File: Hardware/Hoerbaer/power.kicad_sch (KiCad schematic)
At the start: 63 parts, among them J10 Battery 1S Li-Ion, J12 Battery 1S Li-Ion, Q1 DMG3415UQ-7, U12 MAX17048G, U13 TPS61288, U8 MCP73831T-2ACI/OT (4.2V), U9 TPS63001

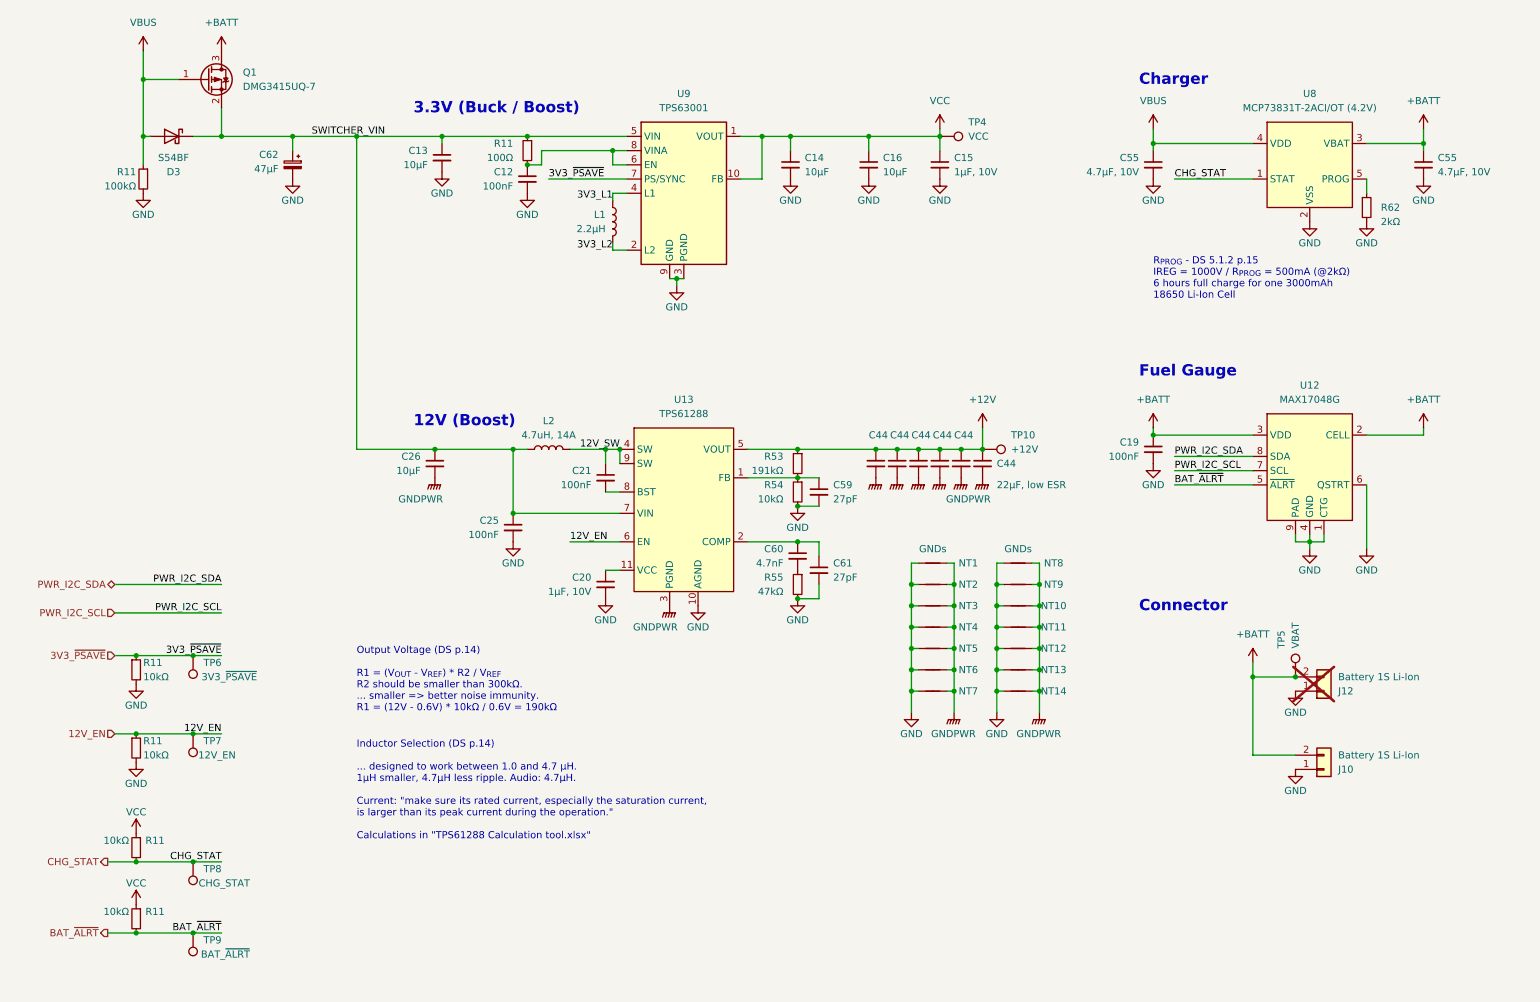
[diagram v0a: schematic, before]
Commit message: WIP new hw rev
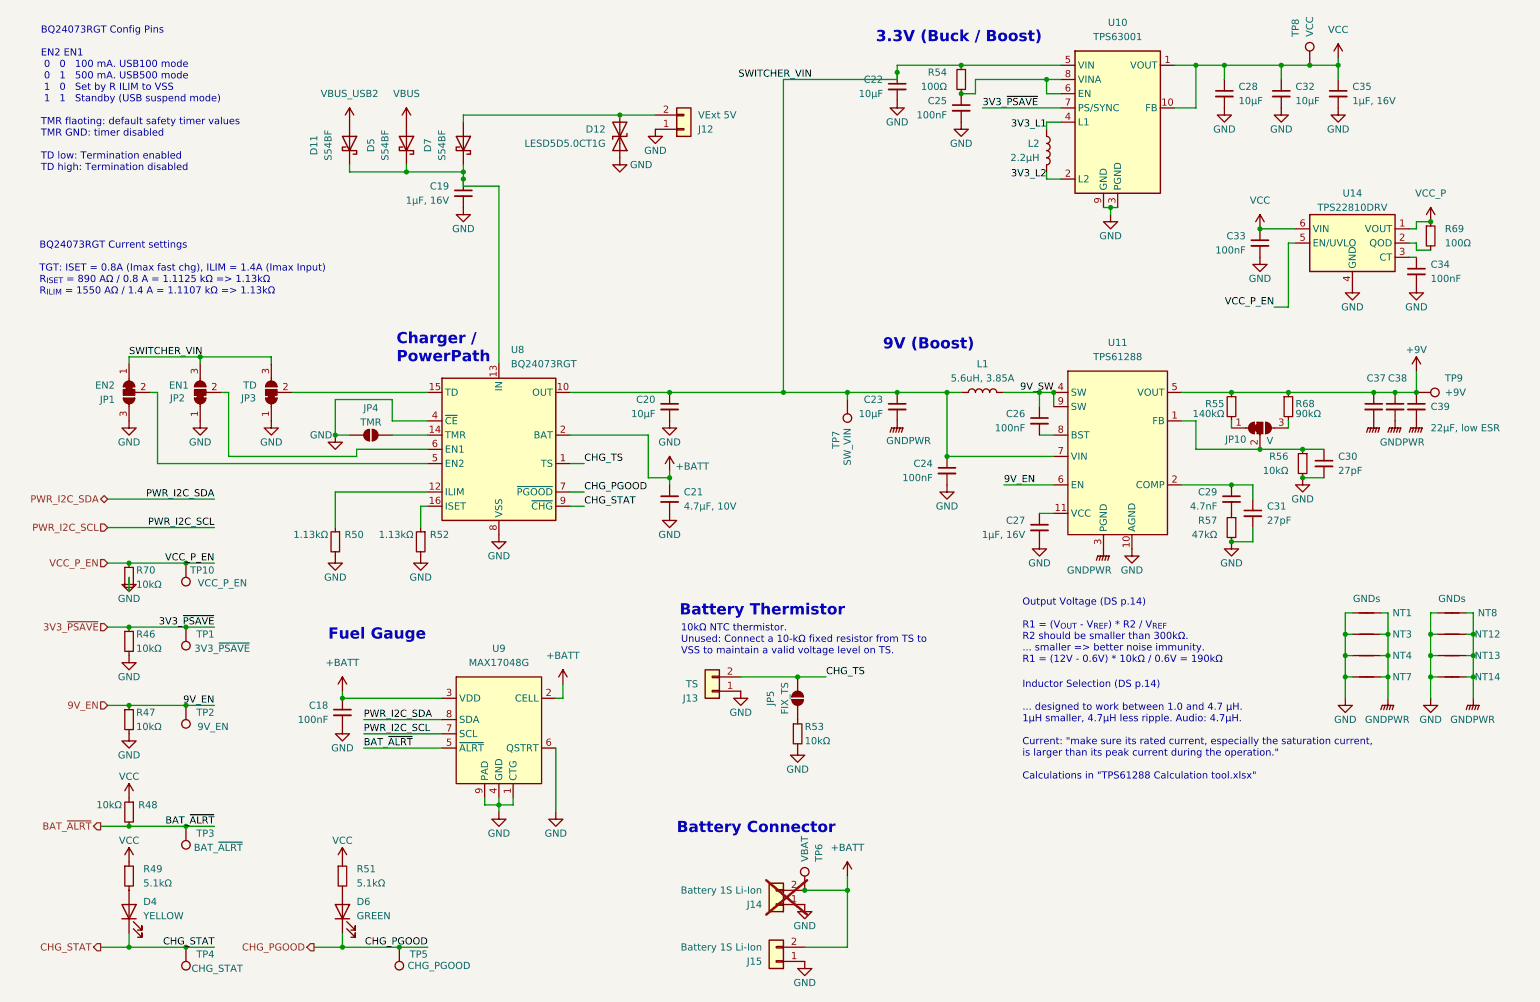
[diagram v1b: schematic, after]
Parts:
- removed C44 (x3): 22µF, low ESR, Capacitor_SMD:C_1210_3225Metric, symbol Device:C_Small
- removed C55: 4.7µF, 10V, Capacitor_SMD:C_0805_2012Metric, symbol Device:C_Small
- removed C62: 47µF, Capacitor_SMD:CP_Elec_6.3x5.9, symbol Device:C_Polarized_Small
- removed NT10, NT11, NT2, NT5, NT6, NT9: GNDs, Baer_Footprints:NetTie-2_Via, symbol Device:NetTie_2
- removed Q1: DMG3415UQ-7, Package_TO_SOT_SMD:SOT-23, symbol Device:Q_PMOS_GSD
- removed R11: 10kΩ, Resistor_SMD:R_0402_1005Metric, symbol Device:R_Small
- removed R11: 100kΩ, Resistor_SMD:R_0402_1005Metric, symbol Device:R_Small
- removed R62: 2kΩ, Resistor_SMD:R_0402_1005Metric, symbol Device:R_Small
- removed U8: MCP73831T-2ACI/OT (4.2V), Package_TO_SOT_SMD:SOT-23-5, symbol Baer_Symbols:MCP73831/2_SOT
- added C19: 1µF, 16V, Capacitor_SMD:C_0402_1005Metric, symbol Device:C_Small
- added C20: 10µF, Capacitor_SMD:C_0805_2012Metric, symbol Device:C_Small
- added C33, C34: 100nF, Capacitor_SMD:C_0402_1005Metric, symbol Device:C_Small
- added D11, D5: S54BF, Baer_Footprints:S54BF, symbol Device:D_Schottky
- added D12: LESD5D5.0CT1G, Diode_SMD:D_SOD-523, symbol Device:D_TVS
- added D4: YELLOW, LED_SMD:LED_0603_1608Metric, symbol Device:LED
- added D6: GREEN, LED_SMD:LED_0603_1608Metric, symbol Device:LED
- added J12: VExt 5V, Connector_Wire:SolderWire-0.5sqmm_1x02_P4.6mm_D0.9mm_OD2.1mm, symbol Connector_Generic:Conn_01x02
- added J13: TS, Connector_PinHeader_2.54mm:PinHeader_1x02_P2.54mm_Vertical, symbol Connector_Generic:Conn_01x02
- added JP1: EN2, Jumper:SolderJumper-3_P1.3mm_Bridged12_RoundedPad1.0x1.5mm, symbol Jumper:SolderJumper_3_Bridged12
- added JP10: V, Jumper:SolderJumper-3_P1.3mm_Bridged12_RoundedPad1.0x1.5mm, symbol Jumper:SolderJumper_3_Bridged12
- added JP2: EN1, Jumper:SolderJumper-3_P1.3mm_Bridged12_RoundedPad1.0x1.5mm, symbol Jumper:SolderJumper_3_Bridged12
- added JP3: TD, Jumper:SolderJumper-3_P1.3mm_Bridged12_RoundedPad1.0x1.5mm, symbol Jumper:SolderJumper_3_Bridged12
- added JP4: TMR, Jumper:SolderJumper-2_P1.3mm_Open_RoundedPad1.0x1.5mm, symbol Jumper:SolderJumper_2_Open
- added JP5: FIX_TS, Jumper:SolderJumper-2_P1.3mm_Open_RoundedPad1.0x1.5mm, symbol Jumper:SolderJumper_2_Open
- added R49, R51: 5.1kΩ, Resistor_SMD:R_0402_1005Metric, symbol Device:R_Small
- added R50, R52: 1.13kΩ, Resistor_SMD:R_0402_1005Metric, symbol Device:R_Small
- added R53, R70: 10kΩ, Resistor_SMD:R_0402_1005Metric, symbol Device:R_Small
- added R68: 90kΩ, Resistor_SMD:R_0402_1005Metric, symbol Device:R_Small
- added R69: 100Ω, Resistor_SMD:R_0402_1005Metric, symbol Device:R_Small
- added TP10: VCC_P_EN, TestPoint:TestPoint_Pad_D1.5mm, symbol Connector:TestPoint
- added TP5: CHG_PGOOD, TestPoint:TestPoint_Pad_D1.5mm, symbol Connector:TestPoint
- added TP7: SW_VIN, TestPoint:TestPoint_Pad_D1.5mm, symbol Connector:TestPoint
- added U14: TPS22810DRV, Package_SON:WSON-6-1EP_2x2mm_P0.65mm_EP1x1.6mm_ThermalVias, symbol Power_Management:TPS22810DRV
- added U8: BQ24073RGT, Package_DFN_QFN:VQFN-16-1EP_3x3mm_P0.5mm_EP1.6x1.6mm, symbol Battery_Management:BQ24073RGT
- C27: renamed from C20; value 1µF, 10V -> 1µF, 16V; LCSC C29266 -> C29266
- C35: renamed from C15; value 1µF, 10V -> 1µF, 16V; LCSC C29266 -> C29266
- L1: renamed from L2; value 4.7uH, 14A -> 5.6uH, 3.85A; footprint Baer_Footprints:L_TDK_SPM12565 -> Inductor_SMD:L_Sunlord_SWPA8040S; LCSC C2048059 -> C96972; MPN SPM12565VT-4R7M-D Copy -> SWPA8040S5R6NT
- R55: renamed from R53; value 191kΩ -> 140kΩ; LCSC C270632 -> C114151; MPN 0402WGF1913TCE -> RC0402FR-07140KL
- TP2: renamed from TP7; value 12V_EN -> 9V_EN
- TP9: renamed from TP10; value +12V -> +9V
- renumbered C19 to C18, C55 to C21, C13 to C22, C26 to C23, C25 to C24, C12 to C25, C21 to C26, C14 to C28, C60 to C29, C59 to C30, C61 to C31, C16 to C32, C44 to C37, C44 to C38, C44 to C39, D3 to D7, J12 to J14, J10 to J15, L1 to L2, R11 to R46, R11 to R47, R11 to R48, R11 to R54, R54 to R56, R55 to R57, TP6 to TP1, TP9 to TP3, TP8 to TP4, TP5 to TP6, TP4 to TP8, U9 to U10, U13 to U11, U12 to U9
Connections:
- net +BATT: now also U8.2 (BAT), U8.3 (BAT)
- net CHG_STAT: now also D4.1 (K), U8.9 (~{CHG})
- net GND: now also C19.2, C20.2, C33.2, C34.2, D12.1 (A1), J12.1 (Pin_1), J13.1 (Pin_1), JP1.3 (B), JP2.1 (A), JP3.1 (A), JP4.1 (A), R50.2, R52.2, R53.2, R70.2, U14.4 (GND), U14.7 (GND), U8.17 (VSS), U8.4 (~{CE}), U8.8 (VSS)
- net SWITCHER_VIN: now also C20.1, JP1.1 (A), JP2.3 (B), JP3.3 (B), TP7.1, U8.10 (OUT), U8.11 (OUT); no longer D7.1 (K)
- net VBUS: now also D5.2 (A); no longer D7.2 (A)
- net VCC: now also C33.1, R49.1, R51.1, U14.6 (VIN)
- net at C30.1, R56.1, U11.1 (FB): now also JP10.2 (C); no longer R55.2
- net +12V renamed +9V
- net +9V: now also R68.1
- net 12V_EN renamed 9V_EN
- net 12V_SW renamed 9V_SW
- new net: R69.2, U14.2 (QOD)
- new net: D12.2 (A2), D7.2 (A), J12.2 (Pin_2)
- new net: C19.1, D11.1 (K), D5.1 (K), D7.1 (K), U8.13 (IN)
- new net: R52.1, U8.16 (ISET)
- new net: JP10.1 (A), R55.2
- new net: JP4.2 (B), U8.14 (TMR)
- new net: JP2.2 (C), U8.6 (EN1)
- new net: C34.1, U14.3 (CT)
- new net: R50.1, U8.12 (ILIM)
- new net: JP3.2 (C), U8.15 (TD)
- new net: JP1.2 (C), U8.5 (EN2)
- new net: JP10.3 (B), R68.2
- new net: D4.2 (A), R49.2
- new net: D6.2 (A), R51.2
- new net: JP5.1 (A), R53.1
- new net CHG_PGOOD: D6.1 (K), TP5.1, U8.7 (~{PGOOD})
- new net CHG_TS: J13.2 (Pin_2), JP5.2 (B), U8.1 (TS)
- new net VBUS_USB2: D11.2 (A)
- new net VCC_P: R69.1, U14.1 (VOUT)
- new net VCC_P_EN: R70.1, TP10.1, U14.5 (EN/UVLO)
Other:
- note added: "10kΩ NTC thermistor. Unused: Connect a 10-kΩ fixed resistor from TS to VSS to maintain a valid voltage level on TS."
- note added: "9V (Boost)"
- note added: "BQ24073RGT Config Pins EN2 EN1 0 0 100 mA. USB100 mode 0 1 500 mA. USB500 mode 1 0 Set by R ILIM to VSS 1 1 Standby (USB suspend mode) TMR flaoting: default safety timer values TMR GND: timer disabled TD low: Termination enabled TD high: Termination disabled"
- note added: "BQ24073RGT Current settings TGT: ISET = 0.8A (Imax fast chg), ILIM = 1.4A (Imax Input) R_{ISET} = 890 AΩ / 0.8 A = 1.1125 kΩ => 1.13kΩ R_{ILIM} = 1550 AΩ / 1.4 A = 1.1107 kΩ => 1.13kΩ"
- note added: "Battery Connector"
- note added: "Battery Thermistor"
- note added: "Charger / PowerPath"
- note removed: "12V (Boost)"
- note removed: "Charger"
- note removed: "Connector"
- note removed: "R_{PROG} - DS 5.1.2 p.15 IREG = 1000V / R_{PROG} = 500mA (@2kΩ) 6 hours full charge for one 3000mAh 18650 Li-Ion Cell"
- moved on the sheet: C18, C21, C22, C23, C24, C25, C26, C27, C28, C29, C30, C31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
